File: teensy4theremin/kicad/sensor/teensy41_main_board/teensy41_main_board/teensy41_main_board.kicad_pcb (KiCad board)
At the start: 2 copper layers, 133.3 x 61 mm, 29 parts, among them J1 LCD_CONTROLS, J10 AUDIO_OUT_EXT, J11 Grounding, J12 SPDIF_IN2, J13 ProtoGrid, J2 LINE_IN, J3 LINE_OUT_BIG, J4 VOL_SENSOR, J5 PITCH_SENSOR, J6 POWER_IN, J7 LINE_OUT_35, J8 EXPR_PED, J9 SPDIF_IN, SW1 SW_Push, U1 Teensy41, U2 TeensyAudioD, U3 PLT133T10W, U4 LD3985M47R_SOT23, U5 LD3985M47R_SOT23

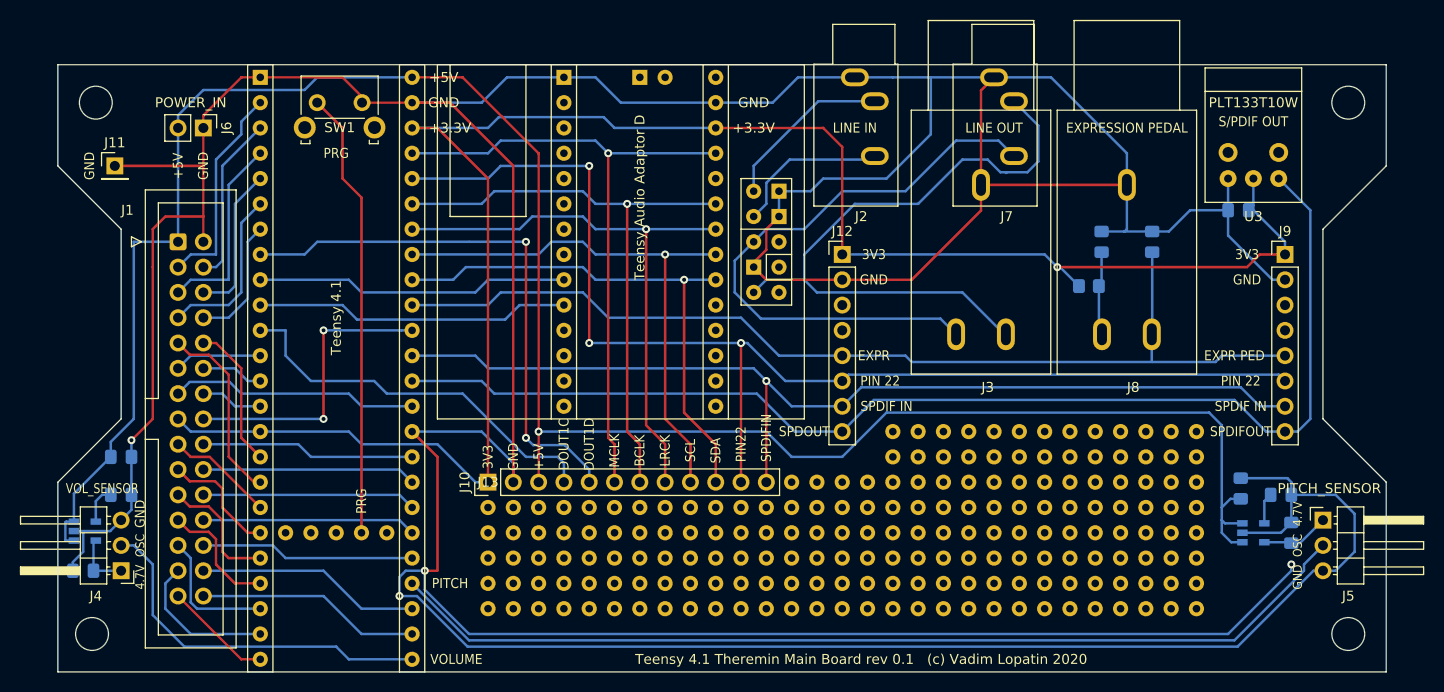
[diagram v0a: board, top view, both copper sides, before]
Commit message: update pcb
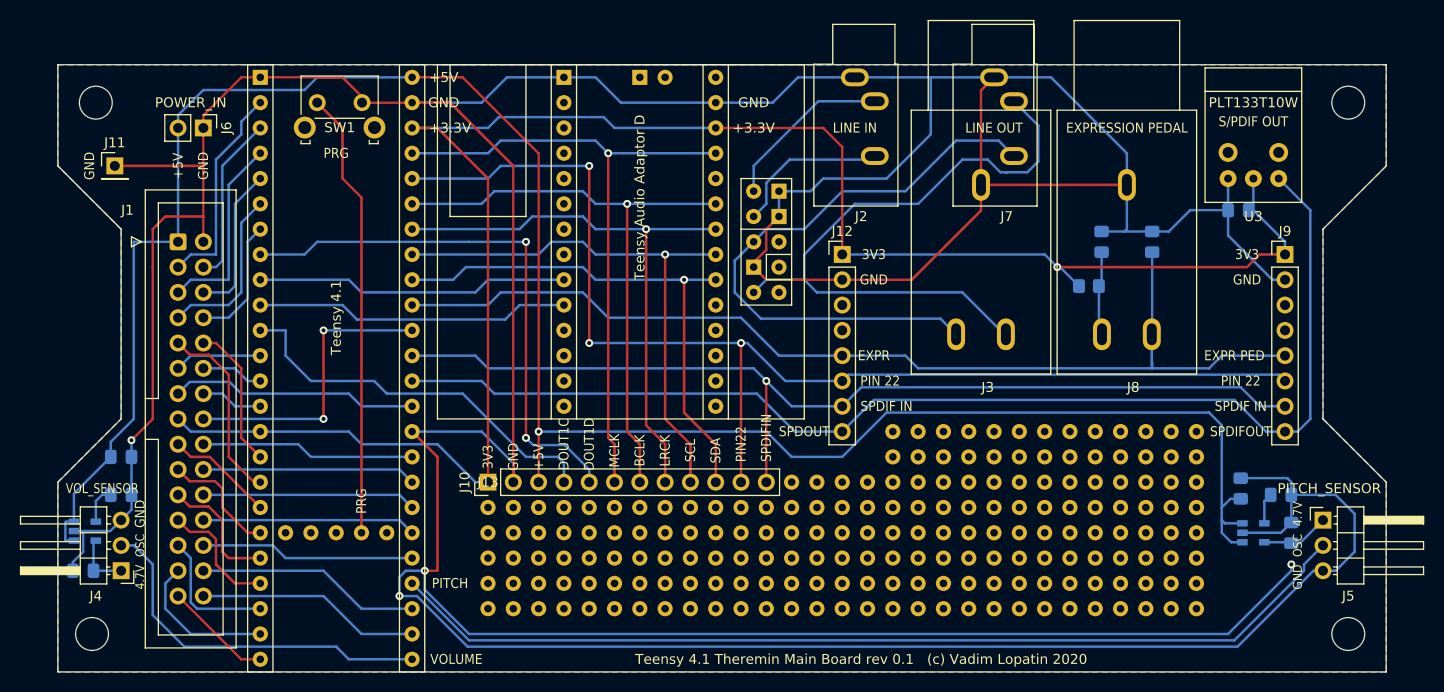
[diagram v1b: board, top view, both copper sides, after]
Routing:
- net /EXPR_PED: track 102.4 -> 104.2 mm
- added copper zone on B.Cu, net GND
- added copper zone on F.Cu, net GND
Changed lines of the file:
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@@
     (thickness 1.6)
     (drawings 139)
-    (tracks 499)
+    (tracks 500)
     (zones 0)
     (modules 29)
@@
   (layers
     (0 F.Cu signal)
-    (31 B.Cu signal)
+    (31 B.Cu signal hide)
     (32 B.Adhes user)
     (33 F.Adhes user)
@@
     (last_trace_width 0.25)
     (trace_clearance 0.2)
-    (zone_clearance 0.508)
+    (zone_clearance 0.3)
     (zone_45_only no)
     (trace_min 0.2)
@@
   (segment (start 142.605 94.065) (end 142.915 94.375) (width 0.25) (layer B.Cu) (net 47))
   (segment (start 142.605 89.535) (end 142.605 94.065) (width 0.25) (layer B.Cu) (net 47))
-  (segment (start 147.915 94.375) (end 147.915 97.115) (width 0.25) (layer B.Cu) (net 48))
-  (segment (start 147.955 97.155) (end 147.915 97.115) (width 0.25) (layer B.Cu) (net 48))
-  (segment (start 154.305 97.155) (end 154.94 96.52) (width 0.25) (layer B.Cu) (net 48))
-  (segment (start 123.825 97.155) (end 154.305 97.155) (width 0.25) (layer B.Cu) (net 48))
-  (segment (start 123.19 96.52) (end 123.825 97.155) (width 0.25) (layer B.Cu) (net 48))
-  (segment (start 154.94 96.52) (end 161.29 96.52) (width 0.25) (layer B.Cu) (net 48))
-  (segment (start 116.84 96.52) (end 123.19 96.52) (width 0.25) (layer B.Cu) (net 48))
   (segment (start 110.49 96.52) (end 116.84 96.52) (width 0.25) (layer B.Cu) (net 48))
   (segment (start 106.68 92.71) (end 110.49 96.52) (width 0.25) (layer B.Cu) (net 48))
@@
   (segment (start 147.955 94.335) (end 147.915 94.375) (width 0.25) (layer B.Cu) (net 48))
   (segment (start 147.955 86.1275) (end 147.955 94.335) (width 0.25) (layer B.Cu) (net 48))
+  (segment (start 154.94 96.52) (end 161.29 96.52) (width 0.25) (layer B.Cu) (net 48))
+  (segment (start 153.67 97.79) (end 154.94 96.52) (width 0.25) (layer B.Cu) (net 48))
+  (segment (start 124.46 97.79) (end 153.67 97.79) (width 0.25) (layer B.Cu) (net 48))
+  (segment (start 123.19 96.52) (end 124.46 97.79) (width 0.25) (layer B.Cu) (net 48))
+  (segment (start 116.84 96.52) (end 123.19 96.52) (width 0.25) (layer B.Cu) (net 48))
+  (segment (start 147.955 97.79) (end 147.955 97.155) (width 0.25) (layer B.Cu) (net 48))
+  (segment (start 147.915 97.75) (end 147.955 97.79) (width 0.25) (layer B.Cu) (net 48))
+  (segment (start 147.915 94.375) (end 147.915 97.75) (width 0.25) (layer B.Cu) (net 48))
   (segment (start 52.705 120.65) (end 64.77 120.65) (width 0.25) (layer B.Cu) (net 49))
   (segment (start 64.77 120.65) (end 68.58 124.46) (width 0.25) (layer B.Cu) (net 49))
@@
   (segment (start 66.675 73.66) (end 66.675 78.74) (width 0.25) (layer F.Cu) (net 67))
   (segment (start 64.135 71.12) (end 66.675 73.66) (width 0.25) (layer F.Cu) (net 67))
+  (zone (net 9) (net_name GND) (layer B.Cu) (hatch edge 0.508)
+    (connect_pads (clearance 0.3))
+    (min_thickness 0.2)
+    (fill yes (arc_segments 32) (thermal_gap 0.508) (thermal_bridge_width 0.508))
+    (polygon
+      (pts
+        (xy 171.45 77.47) (xy 165.1 83.82) (xy 165.1 102.87) (xy 171.45 109.22) (xy 171.45 128.27)
+        (xy 38.1 128.27) (xy 38.1 109.22) (xy 44.45 102.87) (xy 44.45 83.82) (xy 38.1 77.47)
+        (xy 38.1 67.31) (xy 171.45 67.31)
+      )
+    )
+  )
+  (zone (net 9) (net_name GND) (layer F.Cu) (hatch edge 0.508)
+    (connect_pads (clearance 0.3))
+    (min_thickness 0.2)
+    (fill yes (arc_segments 32) (thermal_gap 0.508) (thermal_bridge_width 0.508))
+    (polygon
+      (pts
+        (xy 171.45 77.47) (xy 165.1 83.82) (xy 165.1 102.87) (xy 171.45 109.22) (xy 171.45 128.27)
+        (xy 38.1 128.27) (xy 38.1 109.22) (xy 44.45 102.87) (xy 44.45 83.82) (xy 38.1 77.47)
+        (xy 38.1 67.31) (xy 171.45 67.31)
+      )
+    )
+  )
 )
